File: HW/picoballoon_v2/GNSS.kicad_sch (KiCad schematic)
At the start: 4 parts, among them J3 Conn_Coaxial, U5 MAX-M10S

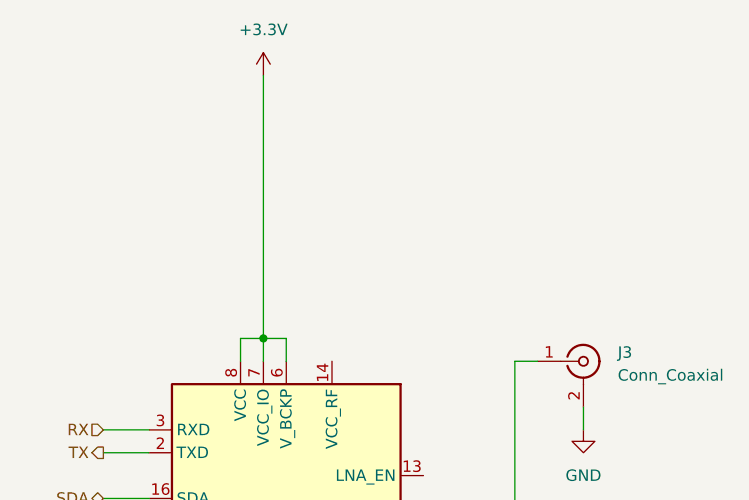
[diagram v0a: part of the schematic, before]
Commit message: little changes in scheme
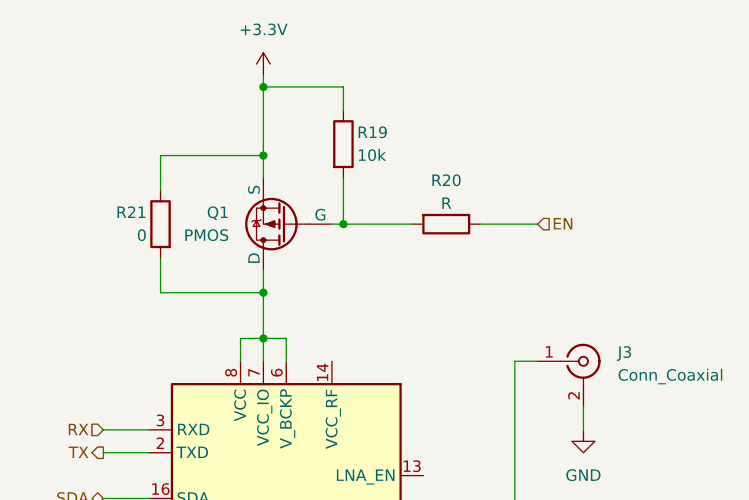
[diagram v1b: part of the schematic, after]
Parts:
- added Q1: PMOS, symbol Simulation_SPICE:PMOS
- added R19: 10k, symbol Device:R
- added R20: R, symbol Device:R
- added R21: 0, symbol Device:R
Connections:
- net +3.3V: now also Q1.3 (S), R19.1, R21.1; no longer U5.6 (V_BCKP), U5.7 (VCC_IO), U5.8 (VCC)
- new net: Q1.1 (D), R21.2, U5.6 (V_BCKP), U5.7 (VCC_IO), U5.8 (VCC)
- new net: Q1.2 (G), R19.2, R20.2
- new net EN: R20.1
